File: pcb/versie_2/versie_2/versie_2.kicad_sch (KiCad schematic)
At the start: 3 parts, among them J2 Conn_01x04_Pin, J3 B4B-PH-SM4-TB__LF__SN_, U1 DFR0654

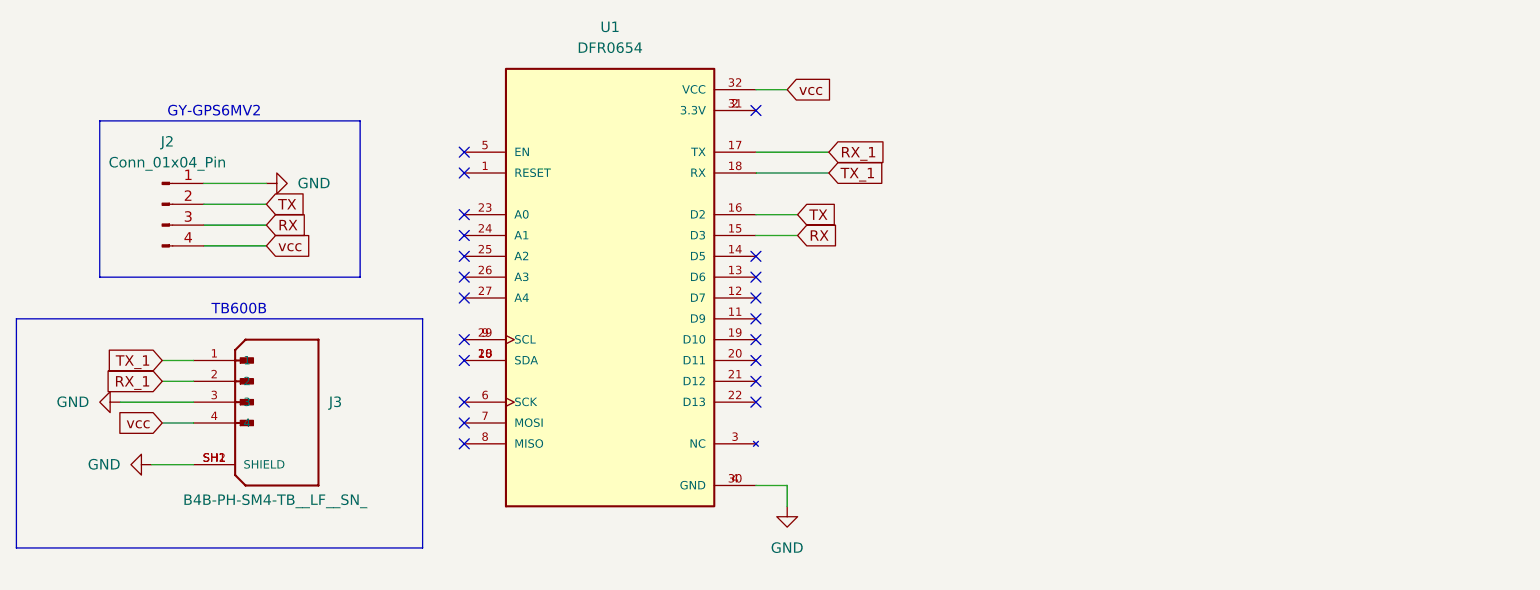
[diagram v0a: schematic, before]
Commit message: PCB_2eversie
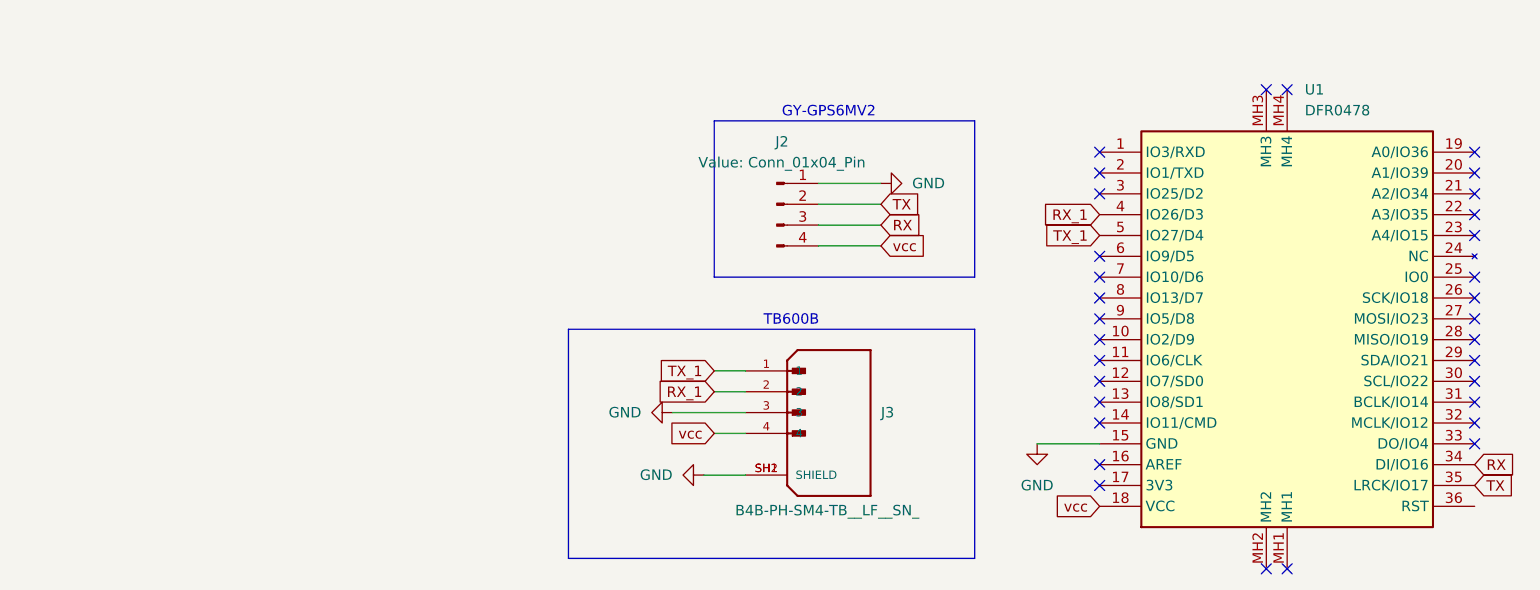
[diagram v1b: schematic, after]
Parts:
- removed U1: DFR0654, warre:MODULE_DFR0654, symbol warre:DFR0654
- added U1: DFR0478, Library:FIREBEETLE_ESP32, symbol footprints:DFR0478
- J2: footprint Connector_PinSocket_2.00mm:PinSocket_1x04_P2.00mm_Horizontal -> Library:GY-GPS6MV2
- J3: footprint Footprints:JST_B4B-PH-SM4-TB__LF__SN_ -> Library:JST_B4B-PH-SM4-TB__LF__SN_
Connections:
- net GND: now also U1.15 (GND)
- net RX: now also U1.34 (DI/IO16)
- net RX_1: now also U1.4 (IO26/D3)
- net TX: now also U1.35 (LRCK/IO17)
- net TX_1: now also U1.5 (IO27/D4)
- net vcc: now also U1.18 (VCC)
- no-connect marks 21 -> 32
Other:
- moved on the sheet: J2, J3
